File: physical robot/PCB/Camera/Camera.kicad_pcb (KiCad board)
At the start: 2 copper layers, 35.8 x 71.3 mm, 101 parts, among them IC1 AMS1117-3.3, IC2 CP2102N-A01-GQFN28, J1 USB_B_Micro, Q1 SS8050-G, Q2 SS8050-G, SW1 SW_Push, SW2 SW_Push, U1 ESP32-WROOM-32, U2 OV5640, U3 ESP32-WROOM-32, X1 CAMERA_OV2640

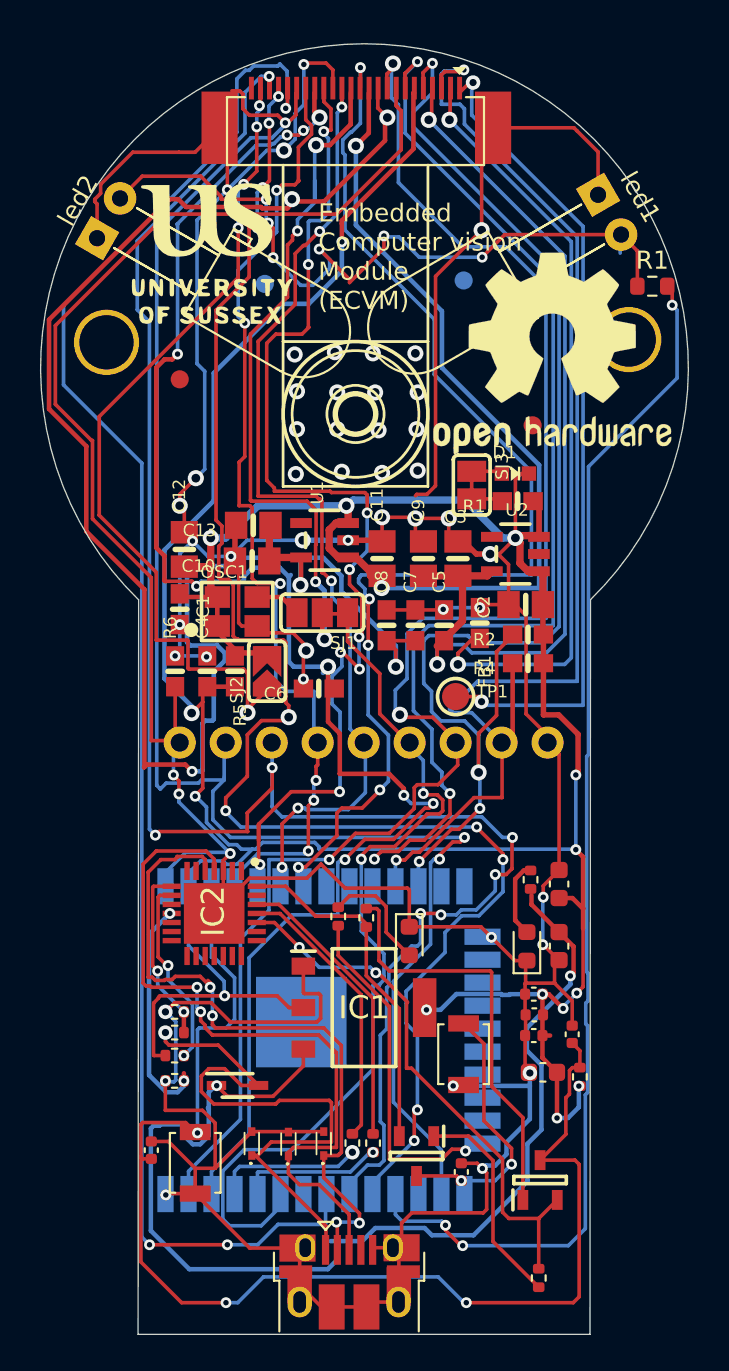
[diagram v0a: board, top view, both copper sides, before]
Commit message: Update Camera.kicad_pcb
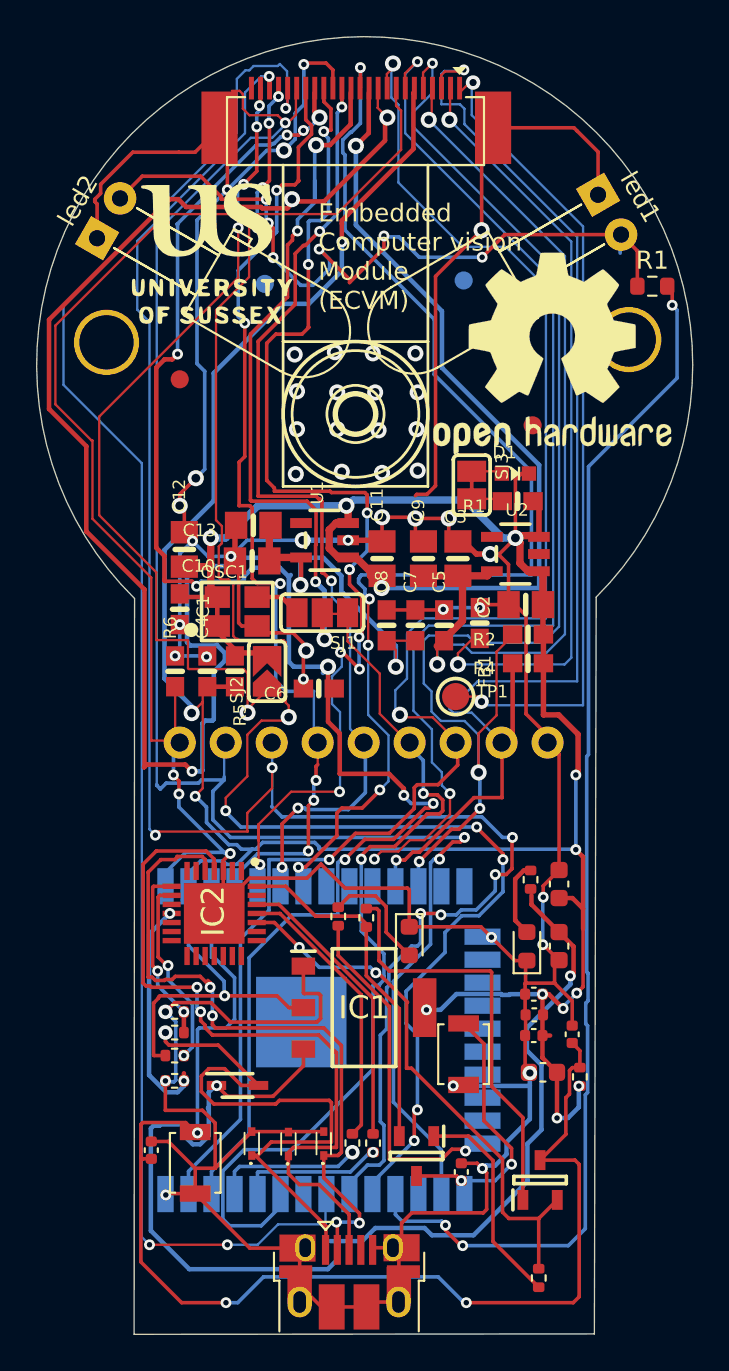
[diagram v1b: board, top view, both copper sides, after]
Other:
- board size 35.8 x 71.3 mm -> 36.2 x 71.7 mm
